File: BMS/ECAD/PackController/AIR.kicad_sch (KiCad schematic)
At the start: 33 parts, among them K401 AIR_N, K402 AIR_P, Q401 DMP4065S-7, Q402 BC846, Q403 DMP4065S-7, Q404 BC846, U401 ADCMP393ARZ

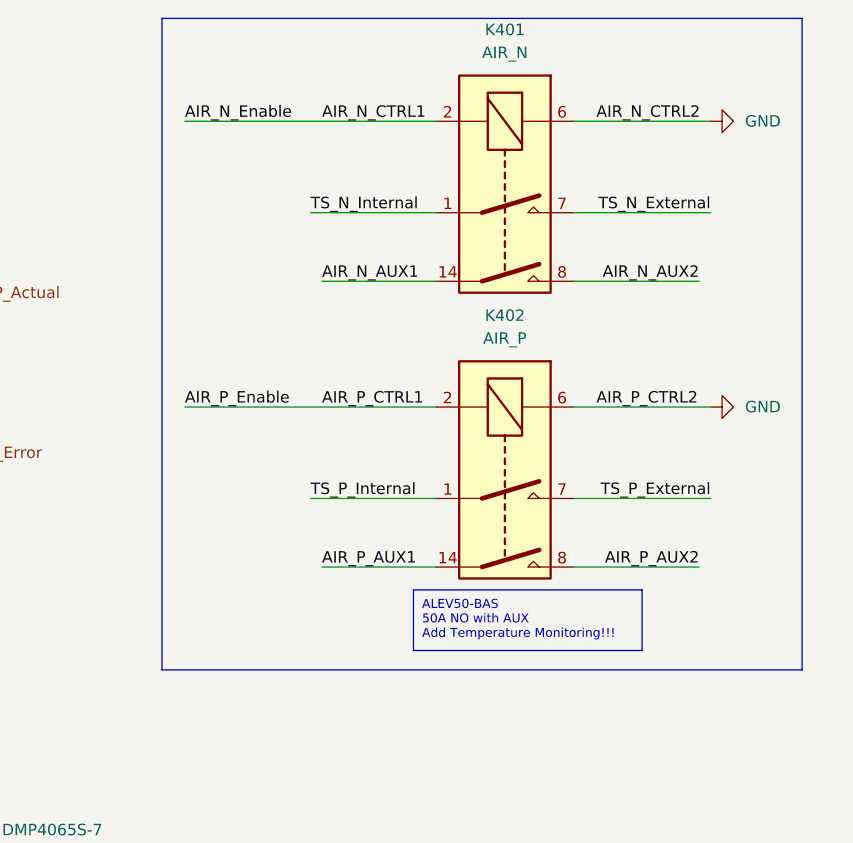
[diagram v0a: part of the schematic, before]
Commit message: yes
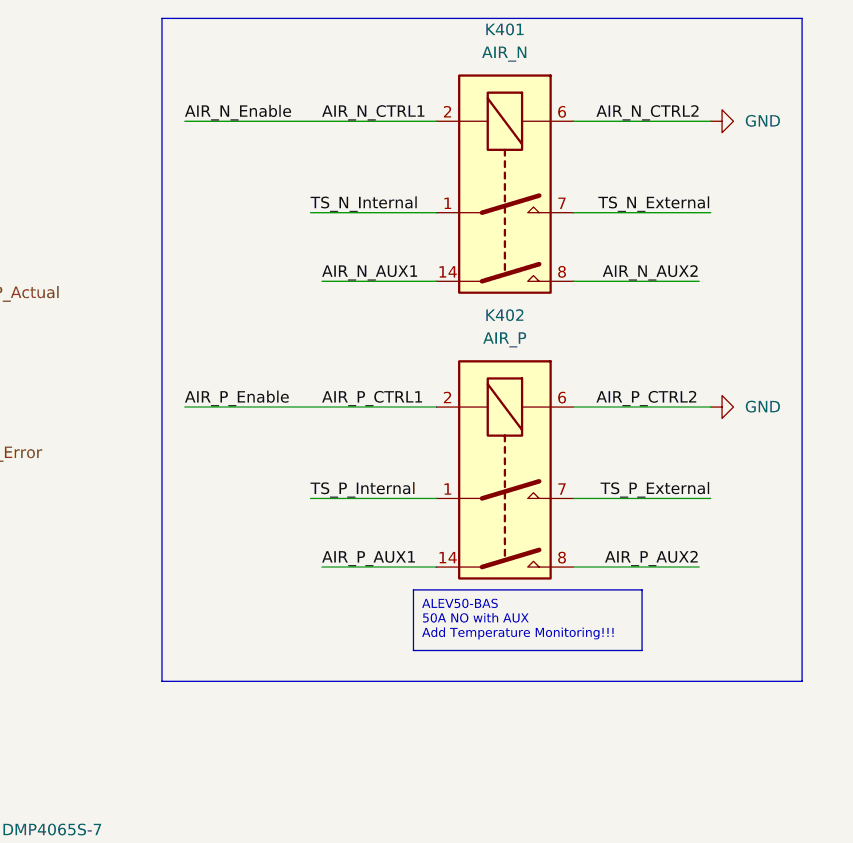
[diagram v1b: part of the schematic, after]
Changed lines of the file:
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@@
 	(rectangle
 		(start 213.36 12.7)
-		(end 284.48 85.09)
+		(end 284.48 86.36)
 		(stroke
 			(width 0)
